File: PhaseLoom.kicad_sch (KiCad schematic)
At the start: 77 parts, among them J1 NC, J1 RF_IN, J2 LO_CLK+90, J2 NC, J3 CLK2, J3 I_OUT, J4 Q_OUT, J5 LO_CLK, Q1 AO3400A, Q2 AO3400A, SW1 USR1, SW2 USR2, SW3 USR3, SW4 USR4, SW5 USR5, T1 50:200, U1 74CBTLV3253PW, U2 ADA4891-2, U3 Si5351A-B-GTR, U5 MIC5504-3.3YM5, Y1 25Mhz

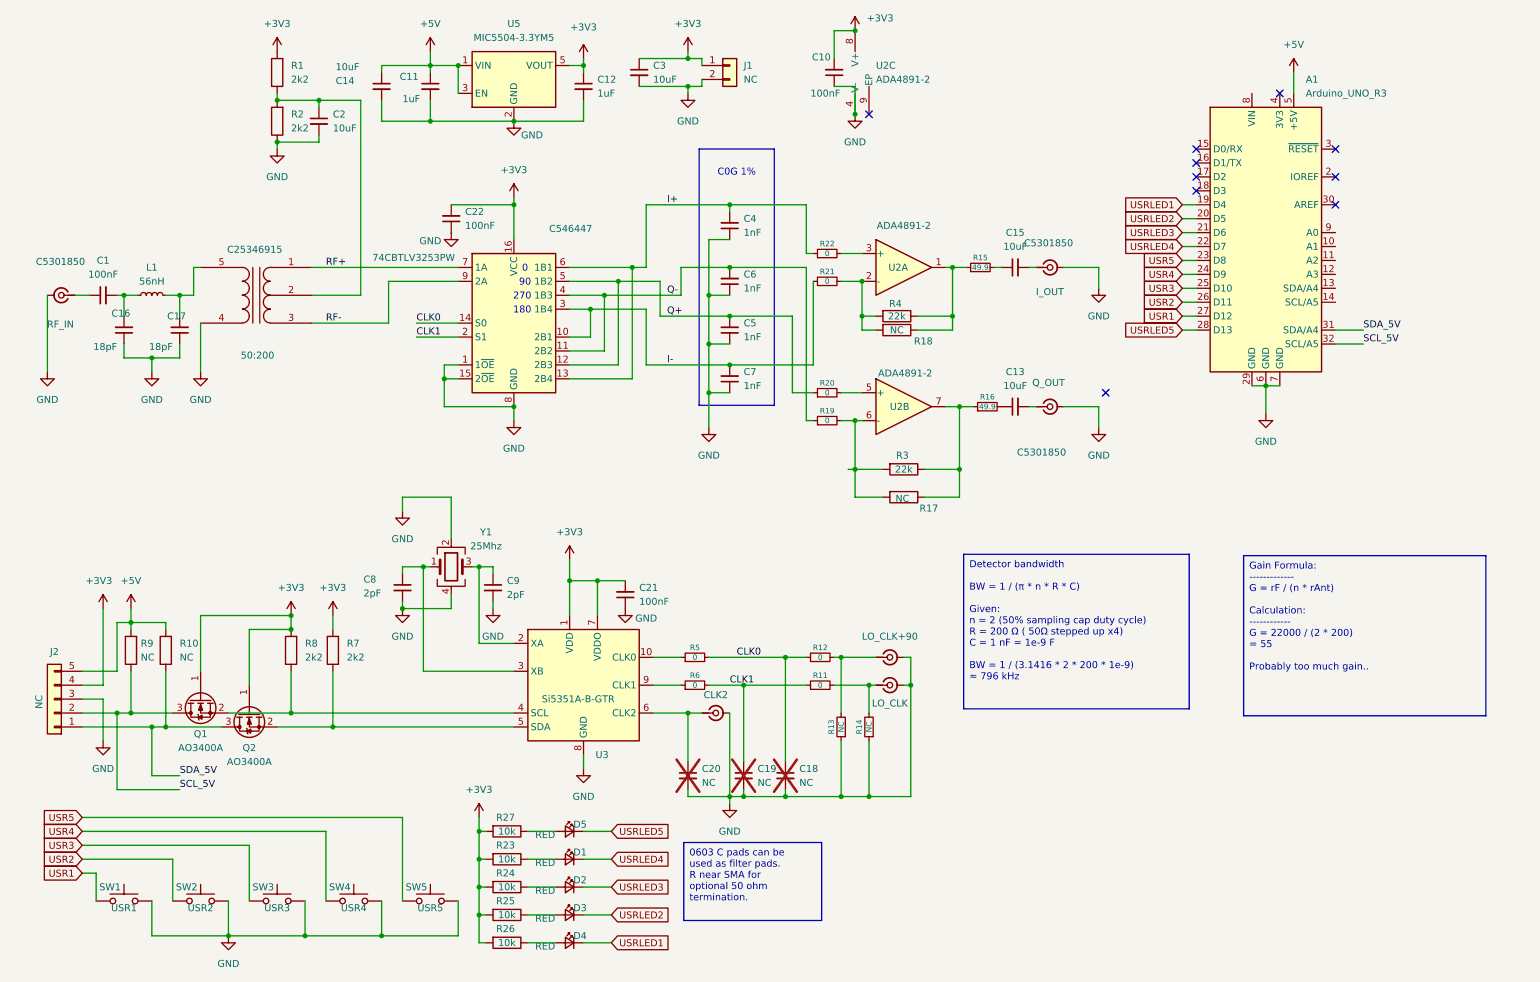
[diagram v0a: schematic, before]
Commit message: Documentation and images
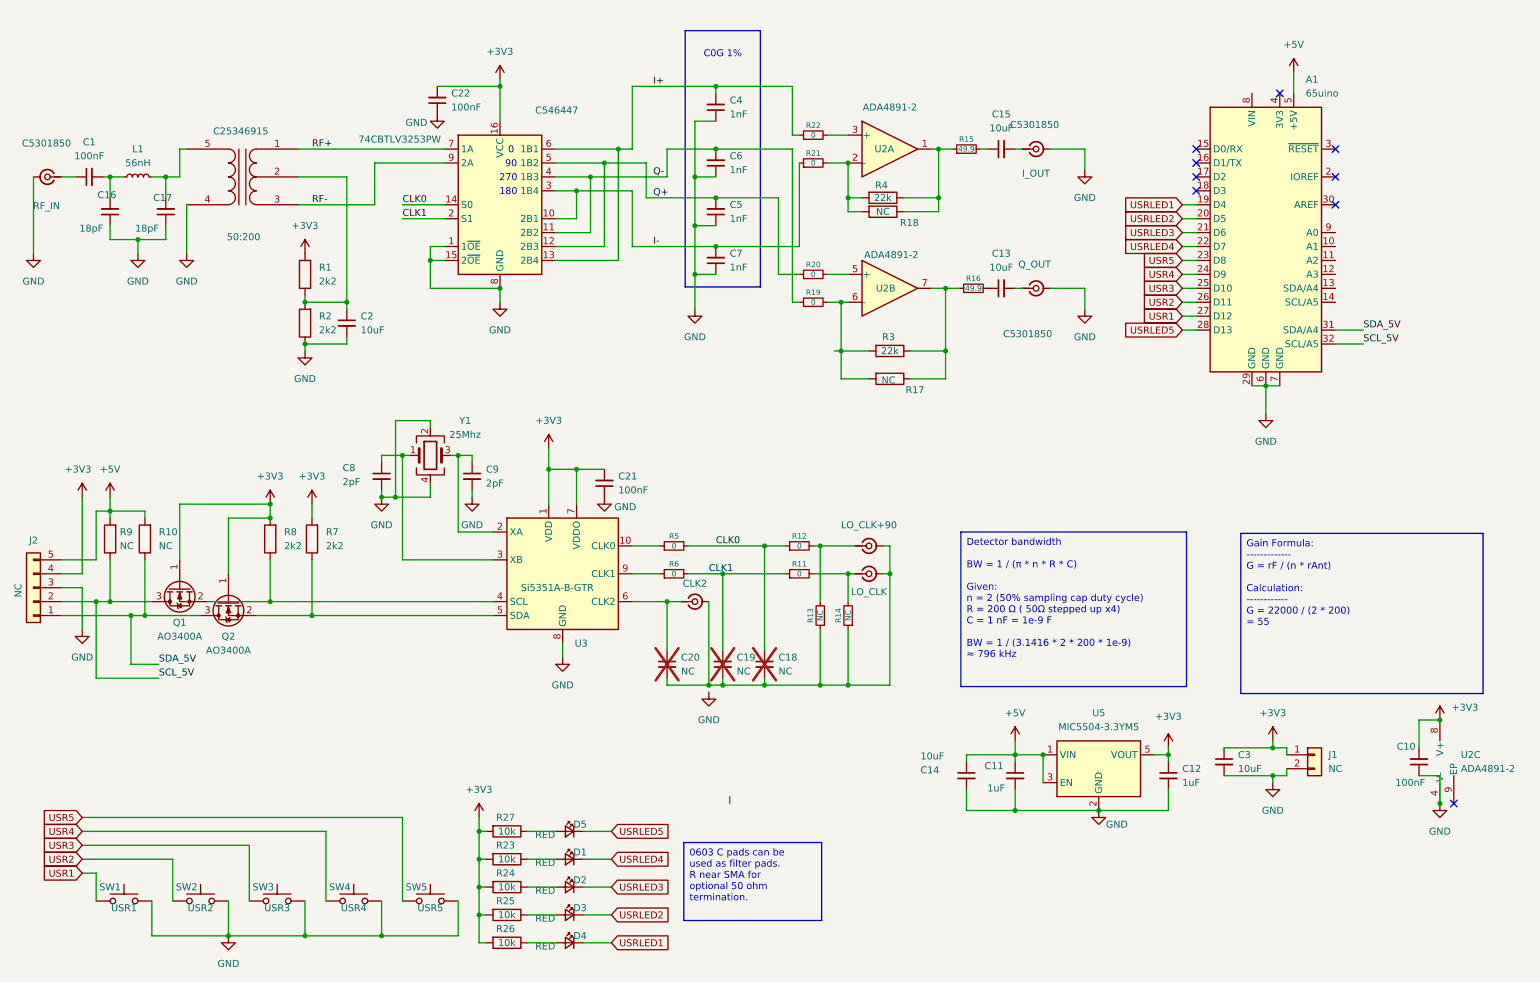
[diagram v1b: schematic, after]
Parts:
- A1: value Arduino_UNO_R3 -> 65uino
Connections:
- net GND: no longer C18.2, C19.2, C20.2, J2.2 (Ext), J3.2 (Ext), J5.2 (Ext), R13.1, R14.1
- new net: C18.2, C19.2, C20.2, J2.2 (Ext), J3.2 (Ext), J5.2 (Ext), R13.1, R14.1
- no-connect marks 10 -> 9
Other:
- moved on the sheet: C1, C10, C11, C12, C13, C14, C15, C16, C17, C18, C19, C2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
